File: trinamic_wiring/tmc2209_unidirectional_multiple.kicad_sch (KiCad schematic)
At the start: 3 parts

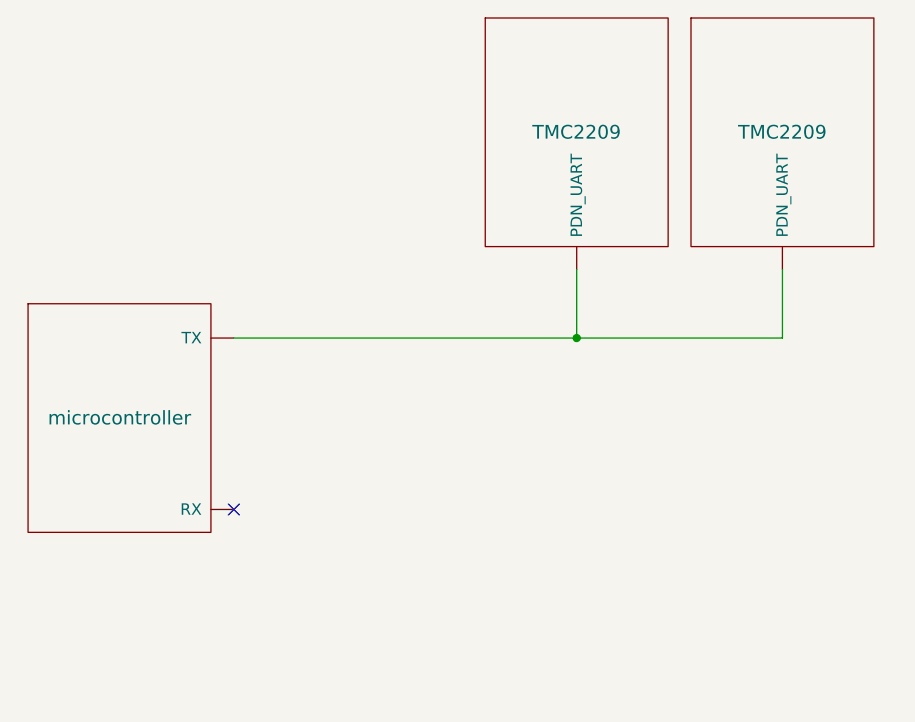
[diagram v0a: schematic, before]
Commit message: Redo schematic symbols
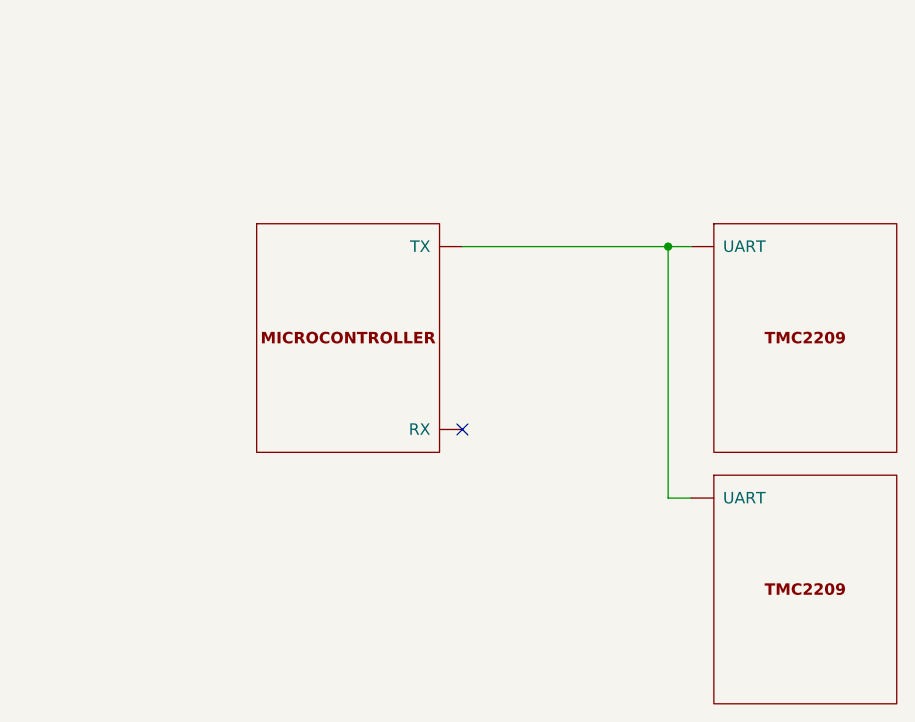
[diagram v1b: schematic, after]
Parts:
- removed TMC? (x2): TMC2209, symbol Janelia:SIMPLIFIED_TMC2209_UART
- removed microcontroller?: microcontroller, symbol Janelia:SIMPLIFIED_MCU_UART
- added MICROCONTROLLER4: DOC_MCU_UART, symbol Janelia:DOC_MCU_UART
- added TMC6 (x2): DOC_TMC2209, symbol Janelia:DOC_TMC2209
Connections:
- new net: MICROCONTROLLER4.1 (TX), TMC6.0 (UART), TMC6.0 (UART)
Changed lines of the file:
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@@
     (company "Janelia Research Campus")
   )
-  (junction (at 138.43 87.63) (diameter 0) (color 0 0 0 0)
+  (junction (at 148.59 77.47) (diameter 0) (color 0 0 0 0)
   )
-  (no_connect (at 100.33 106.68))
-  (wire (pts (xy 138.43 87.63) (xy 161.29 87.63))
+  (no_connect (at 125.73 97.79))
+  (wire (pts (xy 148.59 77.47) (xy 151.13 77.47))
     (stroke (width 0) (type default))
   )
-  (wire (pts (xy 138.43 80.01) (xy 138.43 87.63))
+  (wire (pts (xy 148.59 77.47) (xy 148.59 105.41))
     (stroke (width 0) (type default))
   )
-  (wire (pts (xy 100.33 87.63) (xy 138.43 87.63))
+  (wire (pts (xy 125.73 77.47) (xy 148.59 77.47))
     (stroke (width 0) (type default))
   )
-  (wire (pts (xy 161.29 80.01) (xy 161.29 87.63))
+  (wire (pts (xy 148.59 105.41) (xy 151.13 105.41))
     (stroke (width 0) (type default))
   )
-  (symbol (lib_id "Janelia:SIMPLIFIED_MCU_UART") (at 87.63 96.52 0) (unit 1)
-    (in_bom yes) (on_board yes) (dnp no)
-    (property "Reference" "microcontroller?" (at 87.63 96.52 0) (do_not_autoplace)
+  (symbol (lib_id "Janelia:DOC_MCU_UART") (at 113.03 87.63 0) (unit 1)
+    (in_bom yes) (on_board yes) (dnp no) (fields_autoplaced)
+    (property "Reference" "MICROCONTROLLER4" (at 113.03 68.58 0) (do_not_autoplace)
+      (effects (font (size 1.27 1.27)) hide)
+    )
+    (property "Value" "DOC_MCU_UART" (at 113.03 73.66 0)
       (effects (font (size 1.524 1.524)) hide)
     )
-    (property "Value" "microcontroller" (at 87.63 96.52 0)
-      (effects (font (size 1.524 1.524)))
-    )
-    (property "Footprint" "" (at 85.09 123.19 0)
+    (property "Footprint" "" (at 110.49 114.3 0)
       (effects (font (size 1.524 1.524)) hide)
     )
-    (property "Datasheet" "" (at 87.63 96.52 0)
+    (property "Datasheet" "" (at 113.03 87.63 0)
       (effects (font (size 1.524 1.524)) hide)
+    )
+    (property "Sim.Enable" "0" (at 113.03 71.12 0)
+      (effects (font (size 1.27 1.27)) hide)
     )
     (pin "0")
@@
       (project "trinamic_wiring"
         (path "/e4144788-6304-493f-818e-5d881d3b7418/c8eda2b5-ab13-4033-82d9-875c9fcaf884/13e2a7b5-46df-44bb-8dde-5d79d190b8bf"
-          (reference "microcontroller?") (unit 1)
-        )
-        (path "/e4144788-6304-493f-818e-5d881d3b7418/c8eda2b5-ab13-4033-82d9-875c9fcaf884/e3613d8e-f506-47d6-ad2d-b0f5798d9847"
-          (reference "microcontroller1") (unit 1)
+          (reference "MICROCONTROLLER4") (unit 1)
         )
         (path "/e4144788-6304-493f-818e-5d881d3b7418/c8eda2b5-ab13-4033-82d9-875c9fcaf884/5b0a2695-6b0b-4c82-b9d6-7e19fee75501"
-          (reference "microcontroller3") (unit 1)
-        )
-        (path "/e4144788-6304-493f-818e-5d881d3b7418/c8eda2b5-ab13-4033-82d9-875c9fcaf884/a2ce530e-f5b5-4e3e-9188-e4bc8f84c739"
-          (reference "microcontroller4") (unit 1)
+          (reference "MICROCONTROLLER1") (unit 1)
         )
       )
     )
   )
-  (symbol (lib_id "Janelia:SIMPLIFIED_TMC2209_UART") (at 138.43 64.77 0) (unit 1)
+  (symbol (lib_id "Janelia:DOC_TMC2209") (at 163.83 87.63 0) (unit 1)
     (in_bom yes) (on_board yes) (dnp no) (fields_autoplaced)
-    (property "Reference" "TMC?" (at 138.43 64.77 0) (do_not_autoplace)
+    (property "Reference" "TMC6" (at 163.83 68.58 0)
+      (effects (font (size 1.27 1.27)) hide)
+    )
+    (property "Value" "DOC_TMC2209" (at 163.83 73.66 0)
       (effects (font (size 1.524 1.524)) hide)
     )
-    (property "Value" "TMC2209" (at 138.43 64.77 0)
-      (effects (font (size 1.524 1.524)))
-    )
-    (property "Footprint" "" (at 135.89 91.44 0)
+    (property "Footprint" "" (at 161.29 114.3 0)
       (effects (font (size 1.524 1.524)) hide)
     )
-    (property "Datasheet" "" (at 138.43 64.77 0)
+    (property "Datasheet" "" (at 163.83 87.63 0)
       (effects (font (size 1.524 1.524)) hide)
     )
+    (property "Sim.Enable" "0" (at 163.83 71.12 0)
+      (effects (font (size 1.27 1.27)) hide)
+    )
     (pin "0")
+    (pin "1")
+    (pin "10")
+    (pin "2")
+    (pin "3")
+    (pin "4")
+    (pin "5")
+    (pin "6")
+    (pin "7")
+    (pin "8")
+    (pin "9")
     (instances
       (project "trinamic_wiring"
         (path "/e4144788-6304-493f-818e-5d881d3b7418/c8eda2b5-ab13-4033-82d9-875c9fcaf884/13e2a7b5-46df-44bb-8dde-5d79d190b8bf"
-          (reference "TMC?") (unit 1)
-        )
-        (path "/e4144788-6304-493f-818e-5d881d3b7418/c8eda2b5-ab13-4033-82d9-875c9fcaf884/e3613d8e-f506-47d6-ad2d-b0f5798d9847"
-          (reference "TMC1") (unit 1)
+          (reference "TMC6") (unit 1)
         )
         (path "/e4144788-6304-493f-818e-5d881d3b7418/c8eda2b5-ab13-4033-82d9-875c9fcaf884/5b0a2695-6b0b-4c82-b9d6-7e19fee75501"
-          (reference "TMC4") (unit 1)
-        )
-        (path "/e4144788-6304-493f-818e-5d881d3b7418/c8eda2b5-ab13-4033-82d9-875c9fcaf884/a2ce530e-f5b5-4e3e-9188-e4bc8f84c739"
-          (reference "TMC6") (unit 1)
+          (reference "TMC1") (unit 1)
         )
       )
     )
   )
-  (symbol (lib_id "Janelia:SIMPLIFIED_TMC2209_UART") (at 161.29 64.77 0) (unit 1)
+  (symbol (lib_id "Janelia:DOC_TMC2209") (at 163.83 115.57 0) (unit 1)
     (in_bom yes) (on_board yes) (dnp no) (fields_autoplaced)
-    (property "Reference" "TMC?" (at 161.29 64.77 0) (do_not_autoplace)
+    (property "Reference" "TMC6" (at 163.83 96.52 0)
+      (effects (font (size 1.27 1.27)) hide)
+    )
+    (property "Value" "DOC_TMC2209" (at 163.83 101.6 0)
       (effects (font (size 1.524 1.524)) hide)
     )
-    (property "Value" "TMC2209" (at 161.29 64.77 0)
-      (effects (font (size 1.524 1.524)))
-    )
-    (property "Footprint" "" (at 158.75 91.44 0)
+    (property "Footprint" "" (at 161.29 142.24 0)
       (effects (font (size 1.524 1.524)) hide)
     )
-    (property "Datasheet" "" (at 161.29 64.77 0)
+    (property "Datasheet" "" (at 163.83 115.57 0)
       (effects (font (size 1.524 1.524)) hide)
     )
+    (property "Sim.Enable" "0" (at 163.83 99.06 0)
+      (effects (font (size 1.27 1.27)) hide)
+    )
     (pin "0")
+    (pin "1")
+    (pin "10")
+    (pin "2")
+    (pin "3")
+    (pin "4")
+    (pin "5")
+    (pin "6")
+    (pin "7")
+    (pin "8")
+    (pin "9")
     (instances
       (project "trinamic_wiring"
         (path "/e4144788-6304-493f-818e-5d881d3b7418/c8eda2b5-ab13-4033-82d9-875c9fcaf884/13e2a7b5-46df-44bb-8dde-5d79d190b8bf"
-          (reference "TMC?") (unit 1)
-        )
-        (path "/e4144788-6304-493f-818e-5d881d3b7418/c8eda2b5-ab13-4033-82d9-875c9fcaf884/e3613d8e-f506-47d6-ad2d-b0f5798d9847"
-          (reference "TMC1") (unit 1)
+          (reference "TMC6") (unit 1)
         )
         (path "/e4144788-6304-493f-818e-5d881d3b7418/c8eda2b5-ab13-4033-82d9-875c9fcaf884/5b0a2695-6b0b-4c82-b9d6-7e19fee75501"
-          (reference "TMC5") (unit 1)
-        )
-        (path "/e4144788-6304-493f-818e-5d881d3b7418/c8eda2b5-ab13-4033-82d9-875c9fcaf884/a2ce530e-f5b5-4e3e-9188-e4bc8f84c739"
-          (reference "TMC7") (unit 1)
+          (reference "TMC8") (unit 1)
         )
       )
